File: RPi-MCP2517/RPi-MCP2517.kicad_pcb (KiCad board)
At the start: 2 copper layers, 65 x 56.5 mm, 40 parts, among them J1 Conn_01x06, J2 Conn_01x02, J3 DB9_Female_MountingHoles, P1 CONN_02X20, P2 CONN_01X02, P3 CONN_01X04, P4 CONN_01X04, P8 CONN_01X02, P9 CONN_01X04, U1 MCP2517FD, U2 MCP2562FD, U3 P82B715, U4 SI8641-SOIC, Y1 4MHz

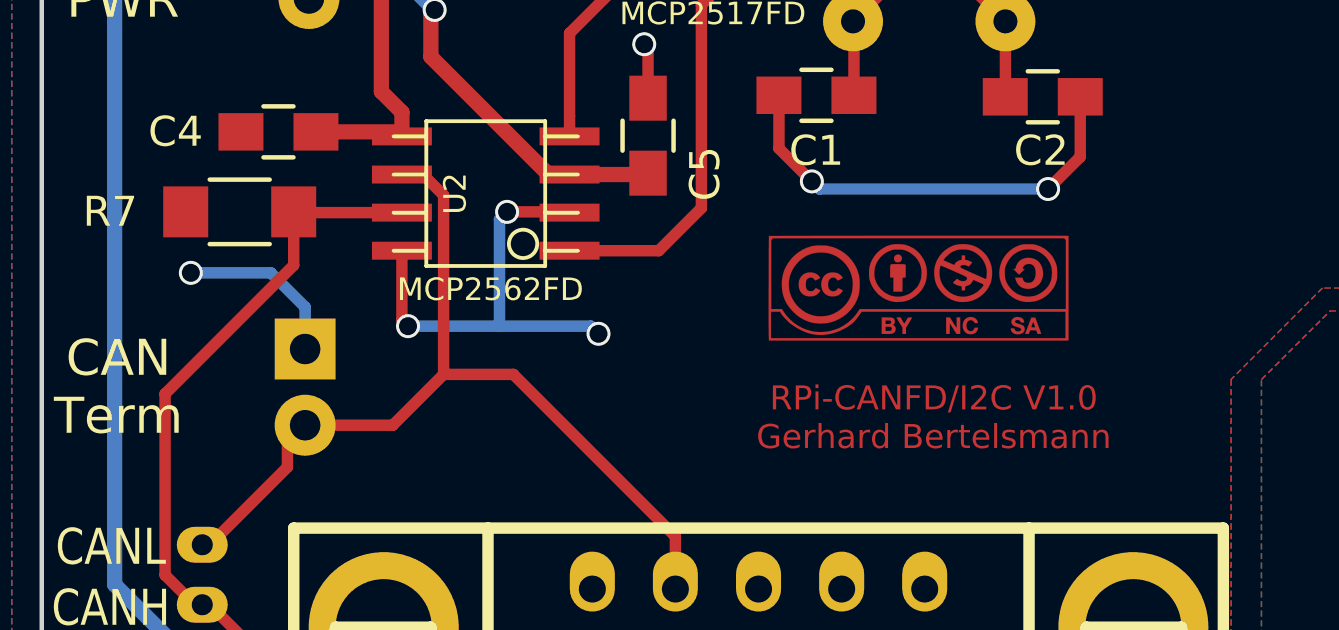
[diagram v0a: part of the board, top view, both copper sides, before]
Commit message: start with fixes for V1.1 part II
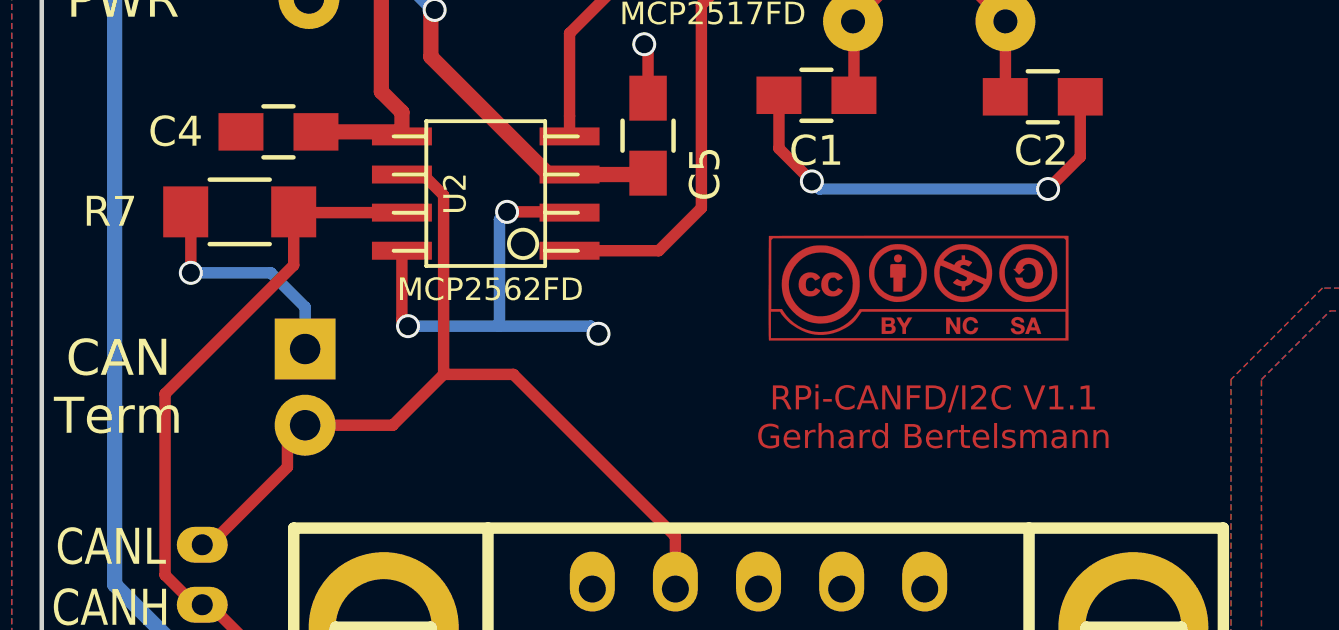
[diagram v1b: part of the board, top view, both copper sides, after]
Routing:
- net Net-(P2-Pad1): track 5.68 -> 7.78 mm
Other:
- board text added: "RPi-CANFD/I2C V1.1 Gerhard Bertelsmann"
- board text removed: "RPi-CANFD/I2C V1.0 Gerhard Bertelsmann"
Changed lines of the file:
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@@
-(kicad_pcb (version 4) (host pcbnew 4.0.7)
+(kicad_pcb (version 4) (host pcbnew 4.0.2+dfsg1-stable)
   (general
     (links 94)
-    (no_connects 1)
-    (area 124.13046 59.3 206.85 142.700001)
+    (no_connects 0)
+    (area 123.82566 59.15 207 142.700001)
     (thickness 1.6)
     (drawings 38)
-    (tracks 420)
+    (tracks 422)
     (zones 0)
     (modules 40)
@@
     (effects (font (size 1.2 1.2) (thickness 0.2)))
   )
-  (gr_text "RPi-CANFD/I2C V1.0\nGerhard Bertelsmann" (at 157.734 109.22) (layer F.Cu)
+  (gr_text "RPi-CANFD/I2C V1.1\nGerhard Bertelsmann" (at 157.734 109.22) (layer F.Cu)
     (effects (font (size 0.8 0.8) (thickness 0.15)))
   )
@@
   (segment (start 136.906 92.71) (end 135.382 92.71) (width 0.508) (layer B.Cu) (net 5))
   (segment (start 135.382 92.71) (end 130.429 87.757) (width 0.508) (layer B.Cu) (net 5))
-  (segment (start 136.779 106.934) (end 136.779 105.537) (width 0.381) (layer B.Cu) (net 27))
+  (segment (start 132.969 102.533) (end 132.969 104.394) (width 0.381) (layer F.Cu) (net 27))
+  (via (at 132.969 104.394) (size 0.8) (drill 0.6) (layers F.Cu B.Cu) (net 27))
+  (segment (start 135.636 104.394) (end 132.969 104.394) (width 0.381) (layer B.Cu) (net 27))
   (segment (start 136.779 105.537) (end 135.636 104.394) (width 0.381) (layer B.Cu) (net 27))
-  (segment (start 135.636 104.394) (end 132.969 104.394) (width 0.381) (layer B.Cu) (net 27))
-  (via (at 132.969 104.394) (size 0.8) (drill 0.6) (layers F.Cu B.Cu) (net 27))
+  (segment (start 136.779 105.537) (end 136.779 106.934) (width 0.381) (layer B.Cu) (net 27))
+  (segment (start 132.969 102.533) (end 132.798 102.362) (width 0.381) (layer F.Cu) (net 27))
   (segment (start 151.09317 94.361) (end 150.368 95.08617) (width 0.381) (layer F.Cu) (net 28))
   (segment (start 150.368 95.08617) (end 149.987 95.46717) (width 0.381) (layer F.Cu) (net 28))
